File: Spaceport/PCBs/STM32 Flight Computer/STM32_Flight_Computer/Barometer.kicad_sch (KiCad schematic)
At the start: 1 part, among them U2 DPS368XTSA1

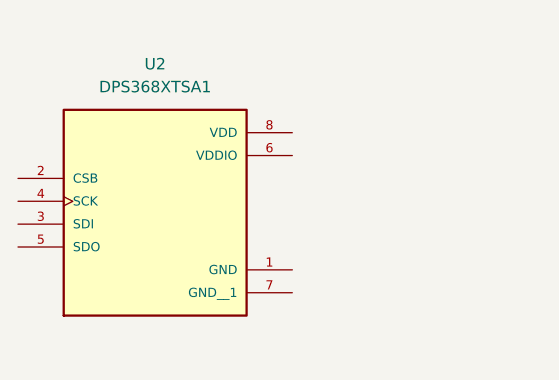
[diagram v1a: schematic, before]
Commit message: Subcircuit Updates
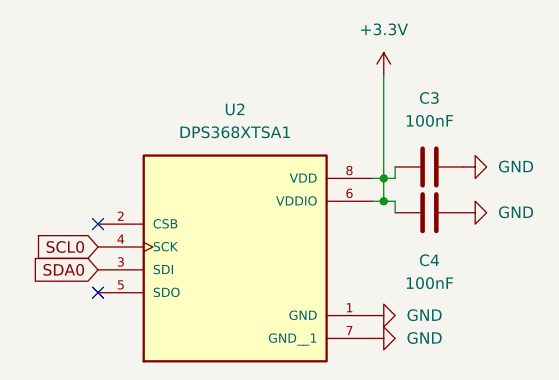
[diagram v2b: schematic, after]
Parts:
- added C3, C4: 100nF, symbol Device:C
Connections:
- net GND: now reaches U2.1 (GND)
- net GND: now also U2.7 (GND__1), C3.2, C4.1
- net SDA0: now reaches U2.3 (SDI)
- net SCL0: now reaches U2.4 (SCK)
- net +3.3V: now reaches U2.6 (VDDIO)
- net +3.3V: now also U2.8 (VDD), C3.1, C4.2
- no-connect marks 0 -> 2
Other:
- moved on the sheet: U2
